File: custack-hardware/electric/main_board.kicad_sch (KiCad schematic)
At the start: 33 parts, among them J2 XH 2.5mmピッチ 2極 オス AWG24, J3 2x15P@2.54mm SMD, J4 PH 2mmピッチ 4極 オス AWG24, J5 PH 2mmピッチ 4極 オス AWG24, J6 PH 2mmピッチ 4極 オス AWG24, Q2 N-ch 30V 4A SOT23F, U1 IN:4.5V-17V, OUT:0.765V-7V,2A

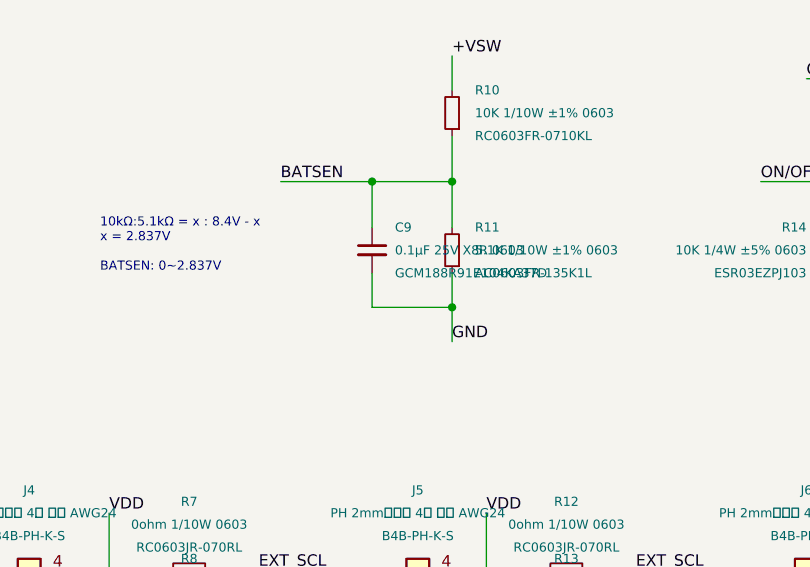
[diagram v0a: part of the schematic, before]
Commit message: complete electric board design
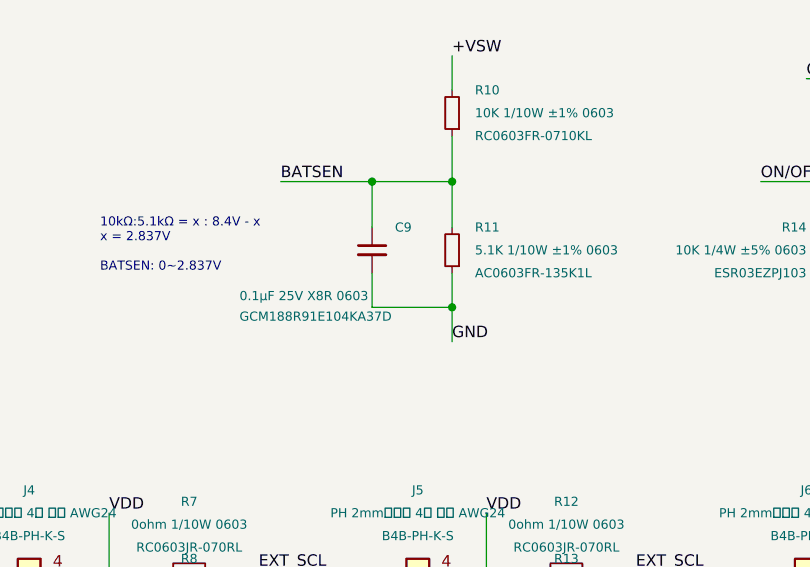
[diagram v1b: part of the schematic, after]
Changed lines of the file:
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@@
 		(in_pos_files yes)
 		(dnp no)
-		(fields_autoplaced yes)
 		(property "Reference" "C9"
 			(at 187.96 102.8762 0)
@@
 		)
 		(property "Value" "0.1µF 25V X8R 0603"
-			(at 187.96 105.4162 0)
+			(at 170.688 110.49 0)
 			(show_name no)
 			(do_not_autoplace no)
@@
 		)
 		(property "型式" "GCM188R91E104KA37D"
-			(at 187.96 107.9562 0)
+			(at 170.688 112.776 0)
 			(show_name no)
 			(do_not_autoplace no)
